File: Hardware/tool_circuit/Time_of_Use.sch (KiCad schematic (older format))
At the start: 2 parts

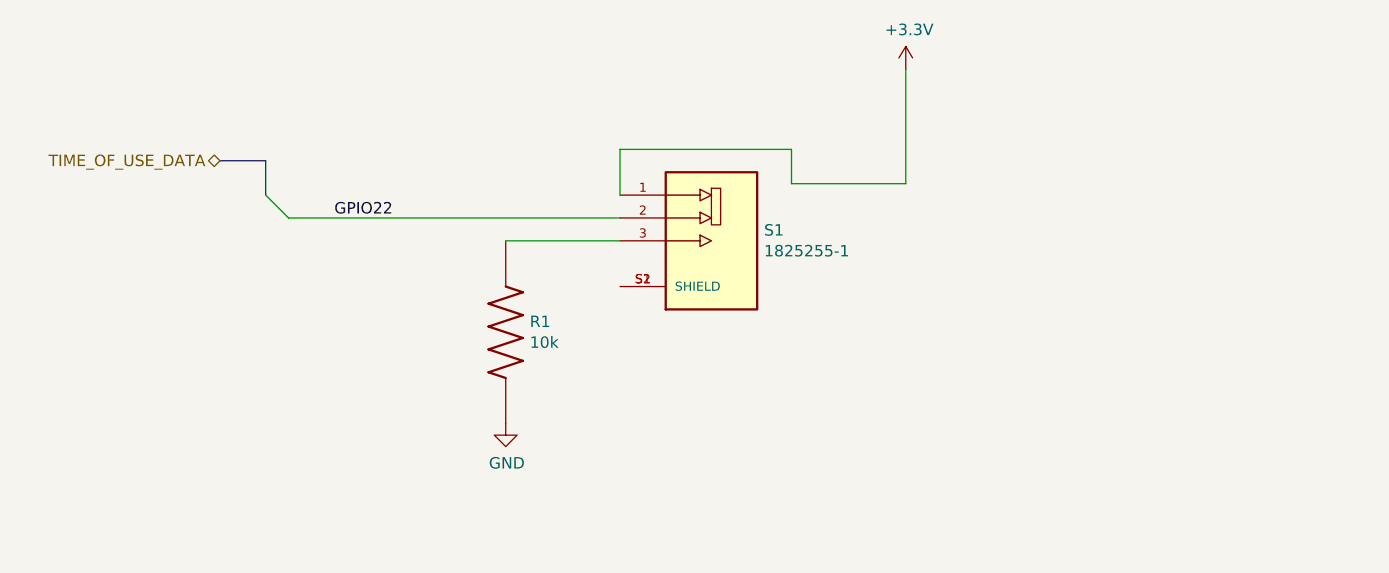
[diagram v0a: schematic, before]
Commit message: layout
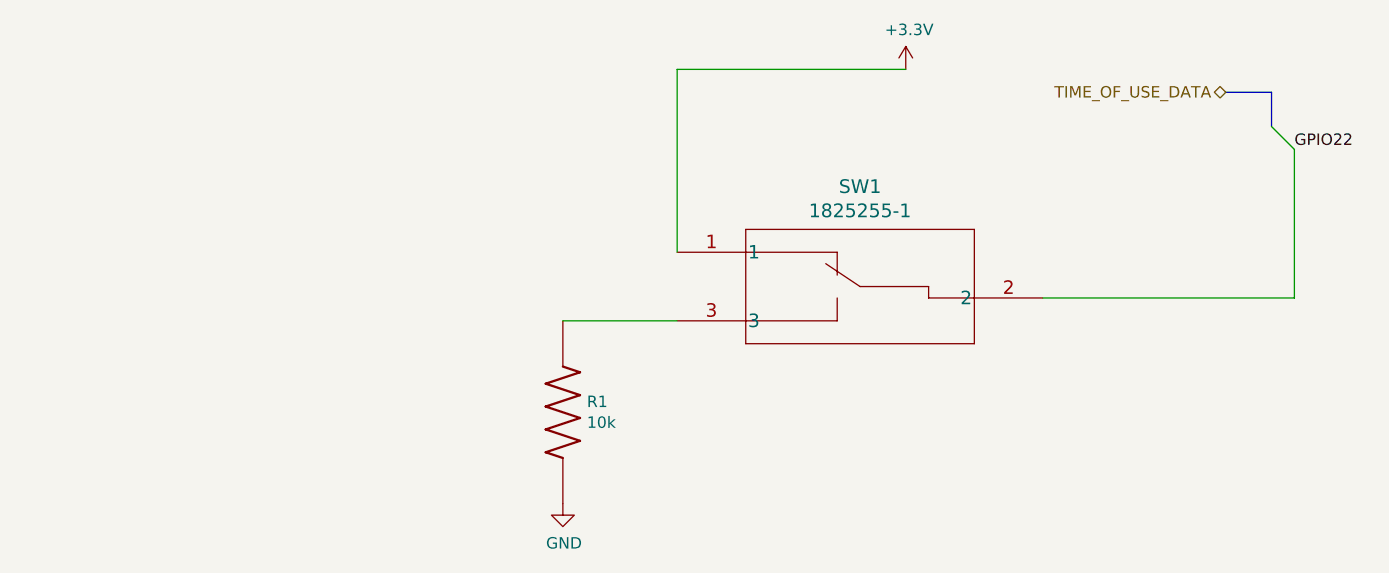
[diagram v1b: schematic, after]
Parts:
- removed S1: 1825255-1, 1825255-1:SW_1825255-1, symbol 1825255-1:1825255-1
- added SW1: 1825255-1, ul_1825255-1:1825255-1, symbol 2021-11-02_22-07-21:1825255-1
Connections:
- net +3V3: now also SW1.1
- net GPIO22: now also SW1.2
- net at R1.1: now also SW1.3
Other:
- moved on the sheet: R1
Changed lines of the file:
@@
 Comment4 ""
 $EndDescr
-Wire Wire Line
-	6650 4000 6150 4000
-$Comp
-L 1825255-1:1825255-1 S1
-U 1 1 61568B03
-P 5800 4250
-F 0 "S1" H 6030 4296 50  0000 L CNN
-F 1 "1825255-1" H 6030 4205 50  0000 L CNN
-F 2 "1825255-1:SW_1825255-1" H 5800 4250 50  0001 L BNN
-F 3 "" H 5800 4250 50  0001 L BNN
-F 4 "1825255-1" H 5800 4250 50  0001 L BNN "Comment"
-	1    5800 4250
-	1    0    0    -1
-$EndComp
-Wire Wire Line
-	6150 4000 6150 3850
-Wire Wire Line
-	6150 3850 5400 3850
-Wire Wire Line
-	5400 3850 5400 4050
-Wire Wire Line
-	6650 3500 6650 4000
 $Comp
 L power:GND #PWR06
 U 1 1 61707039
-P 4900 5050
-F 0 "#PWR06" H 4900 4800 50  0001 C CNN
-F 1 "GND" H 4905 4877 50  0000 C CNN
-F 2 "" H 4900 5050 50  0001 C CNN
-F 3 "" H 4900 5050 50  0001 C CNN
-	1    4900 5050
+P 5150 5400
+F 0 "#PWR06" H 5150 5150 50  0001 C CNN
+F 1 "GND" H 5155 5227 50  0000 C CNN
+F 2 "" H 5150 5400 50  0001 C CNN
+F 3 "" H 5150 5400 50  0001 C CNN
+	1    5150 5400
 	1    0    0    -1
 $EndComp
@@
 	1    0    0    -1
 $EndComp
-Wire Wire Line
-	3950 4150 5400 4150
 Wire Bus Line
-	3850 3900 3850 4050
-Text HLabel 3650 3900 0    50   BiDi ~ 0
+	8250 3600 8250 3750
+Text HLabel 8050 3600 0    50   BiDi ~ 0
 TIME_OF_USE_DATA
 Wire Bus Line
-	3650 3900 3850 3900
+	8050 3600 8250 3600
 Entry Wire Line
-	3850 4050 3950 4150
-Text Label 4150 4150 0    50   ~ 0
+	8250 3750 8350 3850
+Text Label 8350 3850 0    50   ~ 0
 GPIO22
 Wire Wire Line
-	4900 4250 5400 4250
+	5150 4600 5650 4600
 $Comp
 L RNCP1206FTD10K0:RNCP1206FTD10K0 R1
 U 1 1 617867AC
-P 4900 4650
-F 0 "R1" V 4854 4755 50  0000 L CNN
-F 1 "10k" V 4945 4755 50  0000 L CNN
-F 2 "RNCP1206FTD10K0:RESC3115X60N" H 4900 4650 50  0001 L BNN
-F 3 "" H 4900 4650 50  0001 L BNN
-	1    4900 4650
+P 5150 5000
+F 0 "R1" V 5104 5105 50  0000 L CNN
+F 1 "10k" V 5195 5105 50  0000 L CNN
+F 2 "RNCP1206FTD10K0:RESC3115X60N" H 5150 5000 50  0001 L BNN
+F 3 "" H 5150 5000 50  0001 L BNN
+	1    5150 5000
 	0    1    1    0
 $EndComp
+$Comp
+L 2021-11-02_22-07-21:1825255-1 SW1
+U 1 1 6186D287
+P 5650 4300
+F 0 "SW1" H 6450 4587 60  0000 C CNN
+F 1 "1825255-1" H 6450 4481 60  0000 C CNN
+F 2 "ul_1825255-1:1825255-1" H 6450 4440 60  0001 C CNN
+F 3 "" H 5650 4300 60  0000 C CNN
+	1    5650 4300
+	1    0    0    -1
+$EndComp
+Wire Wire Line
+	6650 3500 5650 3500
+Wire Wire Line
+	5650 3500 5650 4300
+Wire Wire Line
+	8350 3850 8350 4500
+Wire Wire Line
+	8350 4500 7250 4500
 $EndSCHEMATC
